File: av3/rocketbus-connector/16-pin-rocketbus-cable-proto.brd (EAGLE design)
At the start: 10.1 x 12.4 mm, 1 part, among them J3 PSAS-USB-FEMALE-CONNECTOR

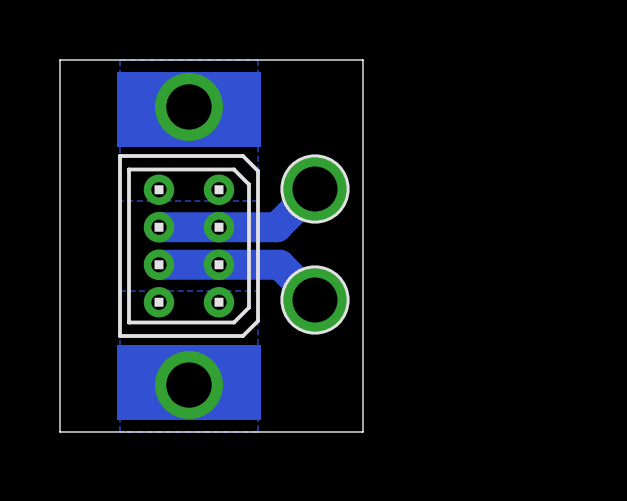
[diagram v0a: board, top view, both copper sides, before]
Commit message: Adding some old rocketbus connectors that we forgot to commit a long time ago.
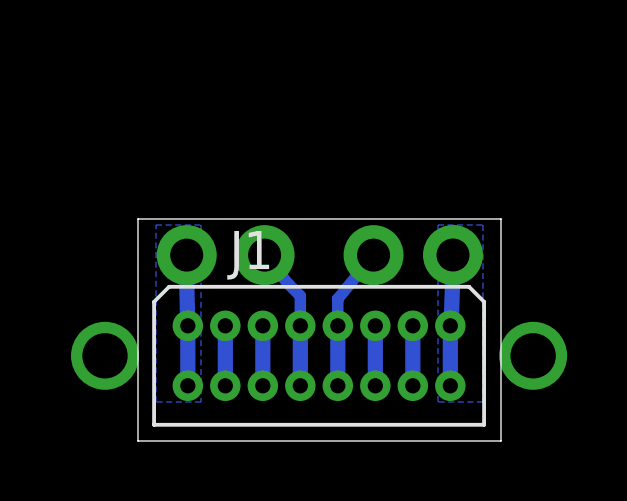
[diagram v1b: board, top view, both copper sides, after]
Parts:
- removed J3: PSAS-USB-FEMALE-CONNECTOR, usb-connector:USB-FEMALE_PKG
- added J1: ROCKETBUS-RECEPTACLE, rocketbus:ROCKETBUS-RECEPTACLE
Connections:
- removed net USB_5V: J3.1, J3.2
- removed net USB_GND: J3.7, J3.8
- removed net USB_H: J3.3, J3.4
- removed net USB_L: J3.5, J3.6
- new net AUX1: J1.AUX1@11, J1.AUX1@12
- new net B+: J1.B+@1, J1.B+@2
- new net B-: J1.B-@15, J1.B-@16
- new net CAN_H: J1.CAN_H@3, J1.CAN_H@4
- new net CAN_L: J1.CAN_L@5, J1.CAN_L@6
- new net S$1: J1.AUX2@13, J1.AUX2@14
- new net USB1_D+: J1.USB_H@7, J1.USB_H@8
- new net USB1_L: J1.USB_L@10, J1.USB_L@9
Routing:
- net USB_L: track 5.73 -> 0.00 mm, vias 1 -> 0
- net USB_H: track 5.69 -> 0.00 mm, vias 1 -> 0
- net USB1_D+: track 0.00 -> 4.81 mm, vias 0 -> 1
- net USB1_L: track 0.00 -> 4.81 mm, vias 0 -> 1
- net B+: track 0.00 -> 4.59 mm, vias 0 -> 1
- net B-: track 0.00 -> 4.36 mm, vias 0 -> 1
- net S$1: track 0.00 -> 2.00 mm
- net CAN_L: track 0.00 -> 2.00 mm
- net CAN_H: track 0.00 -> 2.00 mm
- net AUX1: track 0.00 -> 2.00 mm
- added copper zone on layer 16, net B+
- added copper zone on layer 16, net B-
- removed copper zone on layer 16, net USB_5V
- removed copper zone on layer 16, net USB_GND
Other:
- board size 10.1 x 12.4 mm -> 12.1 x 7.4 mm
- board text added: "B+"
- board text added: "B-"
- board text added: "TOP VIEW (JST CONNECTOR FACING UP)"
- board text added: "USB1_D+"
- board text added: "USB1_D-"
